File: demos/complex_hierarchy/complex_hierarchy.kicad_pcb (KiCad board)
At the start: 2 copper layers, 100.3 x 80 mm, 68 parts, among them P1 CONN_2, P2 CONN_2, P3 CONN_2, P4 CONN_2, P5 CONN_2, P6 CONN_2, Q1 MPSA92, Q2 MPSA42, Q3 MPSA92, Q4 MPSA42, Q5 MPSA92, Q6 MPSA42, Q7 MPSA92, Q8 MPSA42, U1 ICL7660, U2 78L05, U3 LM358N, U4 LM358N

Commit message: Demos update
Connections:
- U1 pad 6: Net-(U1-Pad6) -> unconnected-(U1-Pad6)
- U1 pad 7: Net-(U1-Pad7) -> unconnected-(U1-Pad7)

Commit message: Update demos.
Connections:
- net +12C renamed +12V

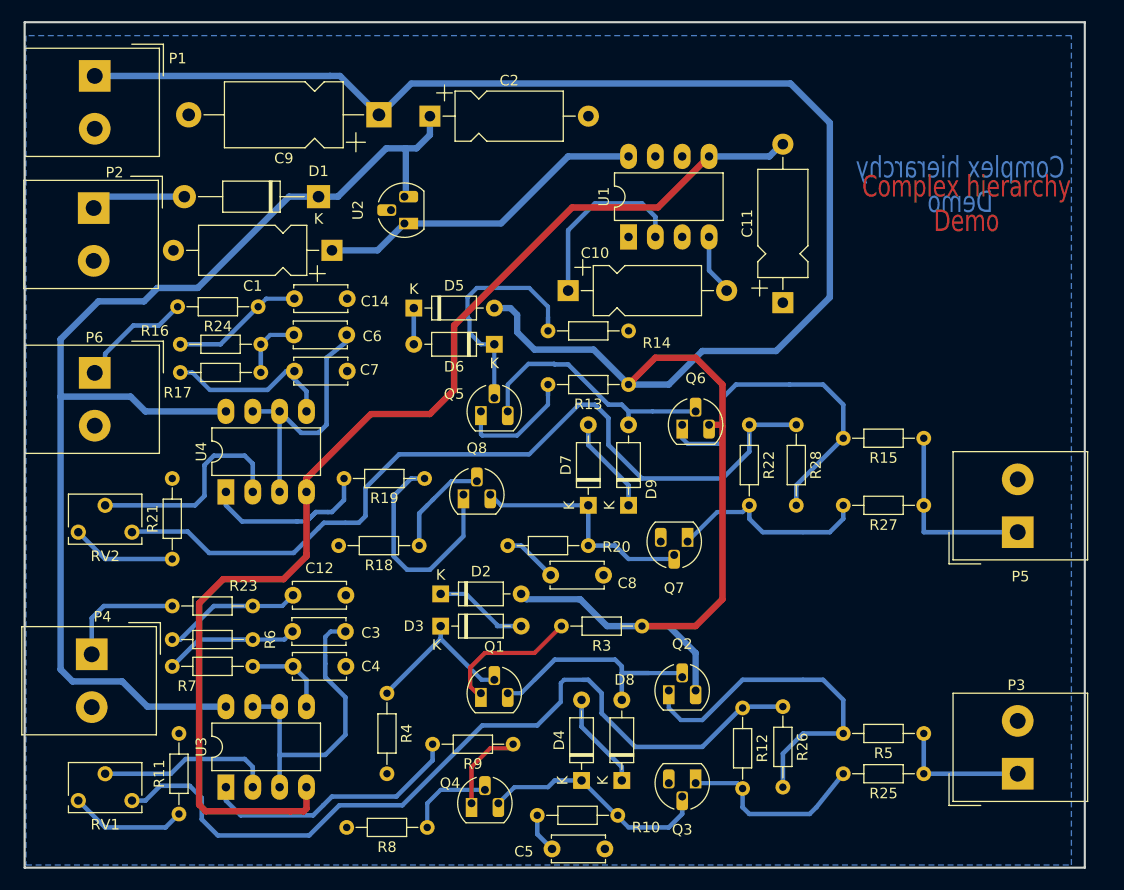
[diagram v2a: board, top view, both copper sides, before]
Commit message: Demos update.
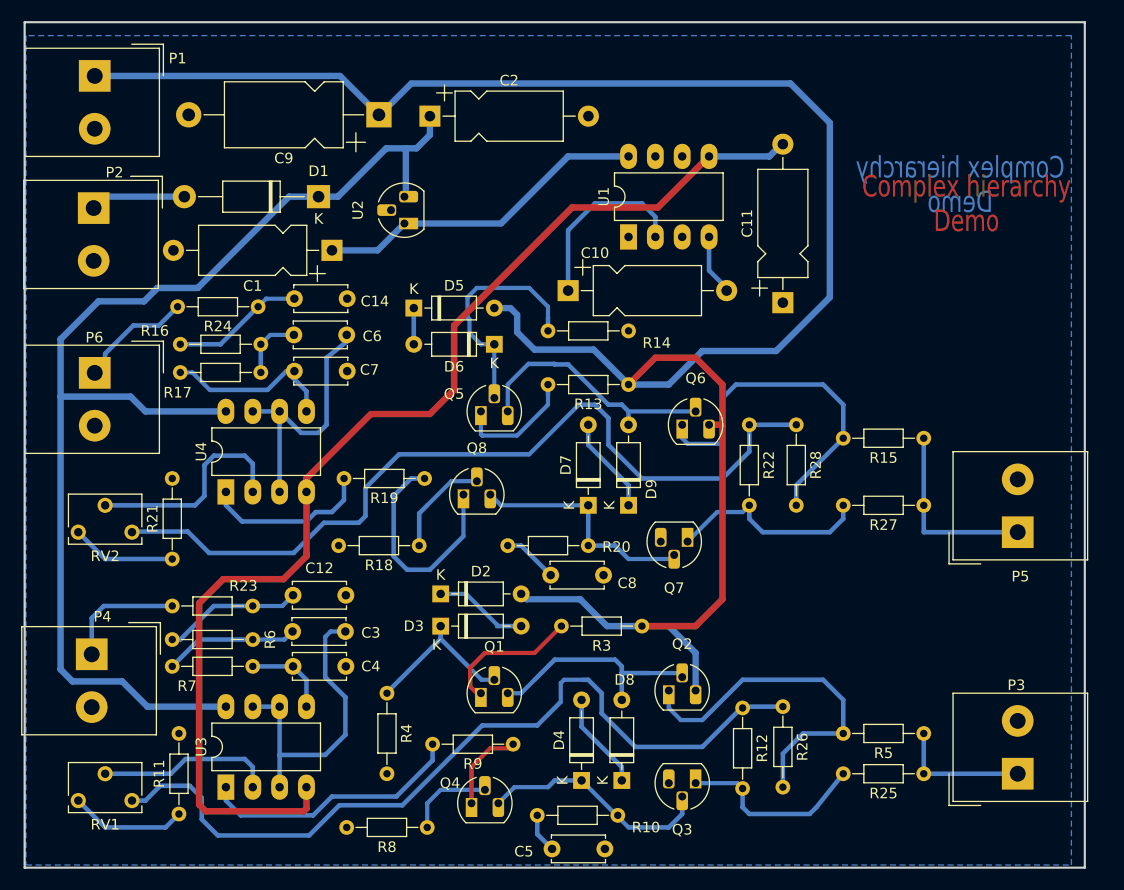
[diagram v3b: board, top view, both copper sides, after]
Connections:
- U1 pad 6: unconnected-(U1-Pad6) -> (no net)
- U1 pad 7: unconnected-(U1-Pad7) -> (no net)
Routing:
- net Net-(R19-Pad2): track 17.2 -> 16.0 mm
- net Net-(D6-Pad1): track 23.0 -> 22.3 mm
